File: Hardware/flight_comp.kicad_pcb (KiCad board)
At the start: 2 copper layers, 86.8 x 48.2 mm, 109 parts, among them IC1 BMP388, J1 Conn_Coaxial, J12 Conn_Coaxial, J2 ARM_SWD_TC2030, J3 XT30, J4 USB_C_Receptacle_USB2.0_16P, J5 Conn_01x02, J6 Conn_01x02, J7 SERVO_CONN_01, J8 SERVO_CONN_02, J9 SERVO_CONN_02, Q2 DMP3013SFV, Q3 CSD17577Q3A, Q4 CSD17577Q3A, Q5 PMBT2222A, SW1 NRST, SW2 BOOT0, U1 STM32F405RGTx, U10 LTC4412, U11 UCC27517A, U12 UCC27517A, U13 LSM6DSO, U2 MAX-M10S, U3 74LVC1GU04, U4 W25Q32JVSS, U5 24LC64, U6 MP2331, U8 USBLC6-2SC6, Y1 8mHz, Y2 32.768 kHz

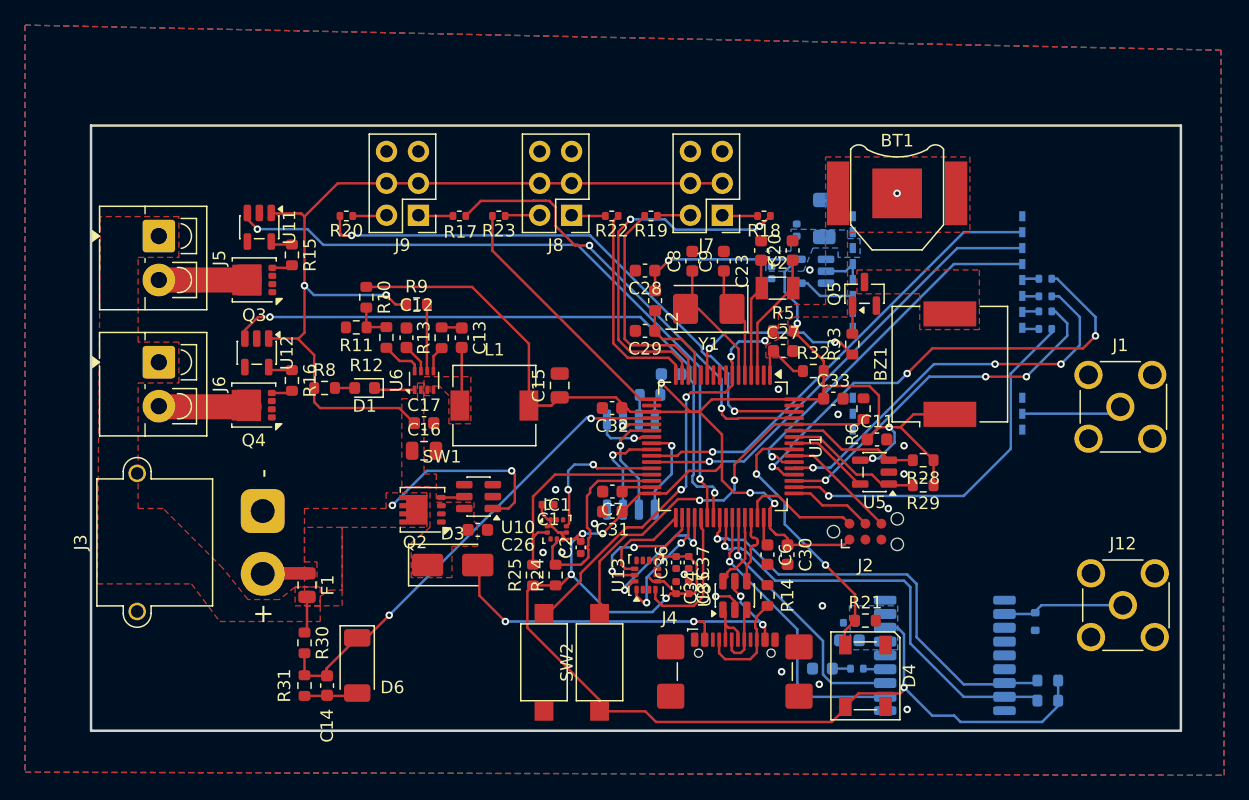
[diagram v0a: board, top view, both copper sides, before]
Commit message: PCB silkscreen, PCB dimensions
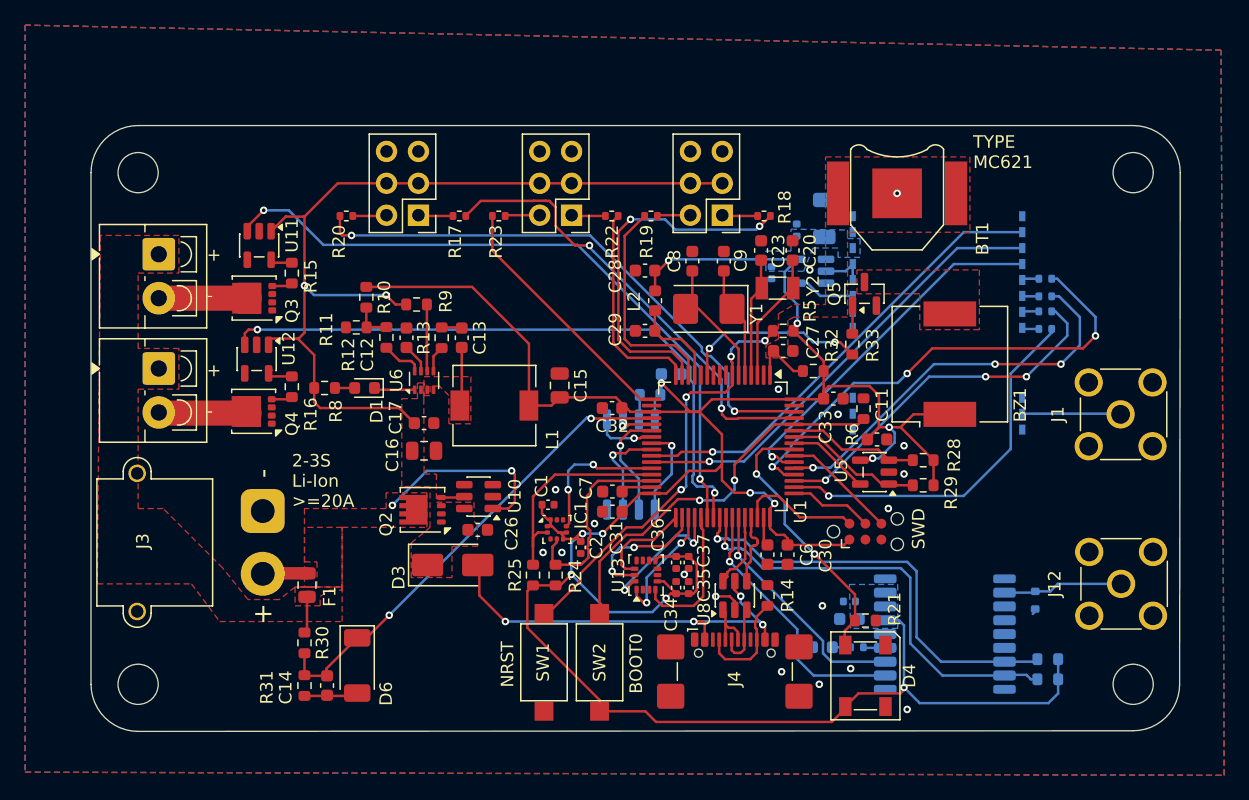
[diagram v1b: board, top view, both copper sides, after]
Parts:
- added H1: MountingHole, MountingHole:MountingHole_3.2mm_M3, F.Cu at (78.0, 126.1)
- added H2: MountingHole, MountingHole:MountingHole_3.2mm_M3, F.Cu at (78.0, 85.3)
- added H3: MountingHole, MountingHole:MountingHole_3.2mm_M3, F.Cu at (157.2, 85.3)
- added H4: MountingHole, MountingHole:MountingHole_3.2mm_M3, F.Cu at (157.2, 126.1)
- BT1: value CR1220 -> MC621
- moved J12 1.71 mm to (156.2, 118.1)
- moved C41 1.70 mm to (134.6, 119.5)
- moved R26 1.70 mm to (150.4, 124.1)
- moved R27 1.70 mm to (150.4, 125.7)
- moved U2 1.70 mm to (142.2, 122.1)
- moved C42 1.70 mm to (134.6, 120.9)
- moved D5 1.70 mm to (149.4, 119.4)
- moved R48 1.70 mm to (135.2, 123.2)
- moved TX4 1.70 mm to (132.4, 123.2)
- moved U11 1.45 mm to (87.6, 91.2)
- moved Q3 1.45 mm to (87.2, 95.3)
- moved R15 1.45 mm to (90.2, 93.3)
- moved J5 1.45 mm to (79.6, 91.8)
- moved J1 0.60 mm to (156.2, 104.6)
- moved R16 0.50 mm to (90.2, 102.4)
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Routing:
- net GPS_TX: track 23.0 -> 21.1 mm
- net GPS_RX: track 20.6 -> 18.9 mm
- net Net-(D5-A2): track 9.72 -> 10.9 mm
- net PYRO_2: track 51.9 -> 50.9 mm
- net PYRO_1: track 53.6 -> 54.3 mm
- net GND: track 6.65 -> 6.93 mm, vias 17 -> 18
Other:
- board size 86.8 x 48.2 mm -> 86.7 x 48.2 mm
- board text added: "+ -"
- board text added: "2-3S Li-Ion >=20A"
- board text added: "BOOT0"
- board text added: "GND VCC S2 S1"
- board text added: "GND VCC S3 S4"
- board text added: "GND VCC S5 S6"
- board text added: "NRST"
- board text added: "PYRO1"
- board text added: "PYRO2"
- board text added: "SWD"
- board text added: "TYPE MC621"
